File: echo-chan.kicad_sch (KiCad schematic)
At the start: 50 parts, among them J1 SJ1-3533NS, J2 USB_B, SW1 SW_Push, T1 Transformer_1P_1S, U1 JAMMA, U2 JAMMA, U3 AT90USB1286, U4 HD15, U6 THS7374, Y1 16MHz

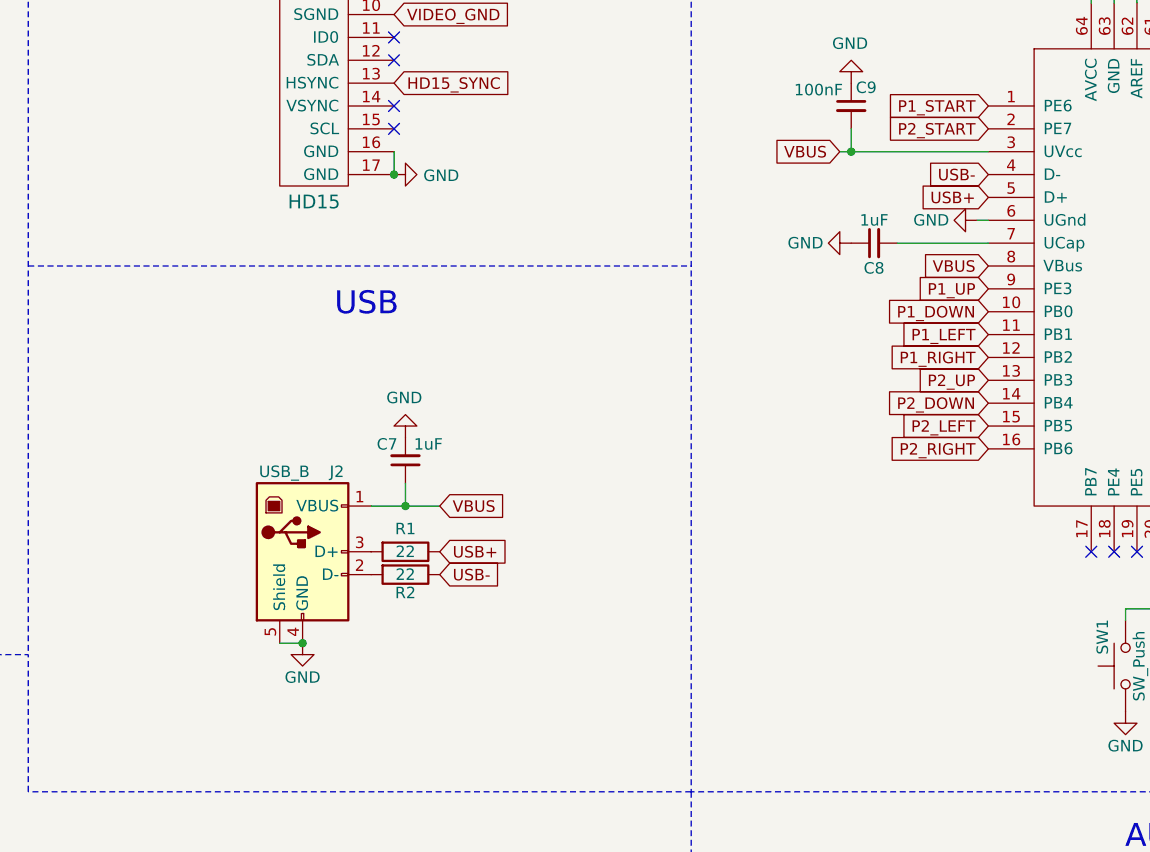
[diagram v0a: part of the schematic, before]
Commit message: [PCB] Routing done
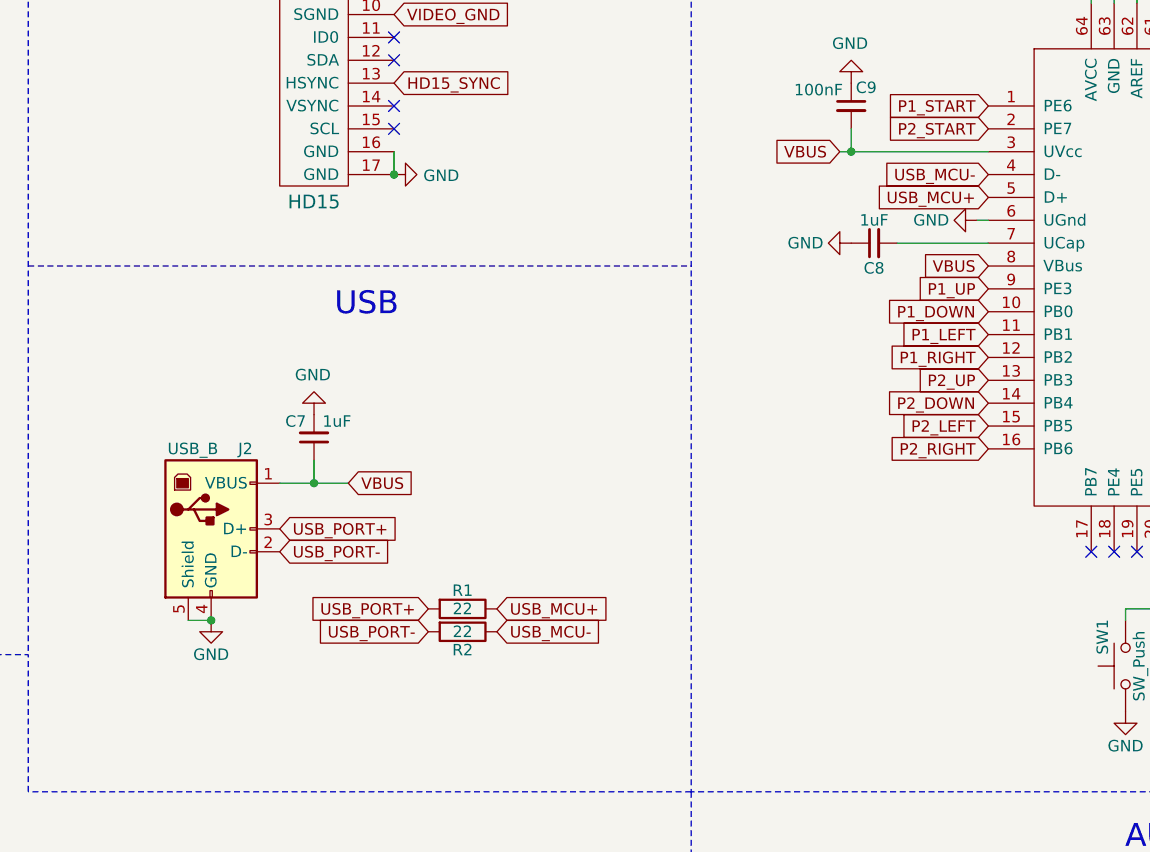
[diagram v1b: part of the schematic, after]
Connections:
- net USB_PORT+: now reaches J2.3 (D+), R1.2
- net USB_PORT-: now reaches J2.2 (D-), R2.2
- net USB+ renamed USB_MCU+
- net USB- renamed USB_MCU-
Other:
- moved on the sheet: C7, J2, R1, R2
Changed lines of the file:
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@@
 	)
 	(junction
-		(at 125.73 118.11)
+		(at 115.57 115.57)
 		(diameter 0)
 		(color 0 0 0 0)
@@
 	)
 	(junction
-		(at 137.16 102.87)
+		(at 127 100.33)
 		(diameter 0)
 		(color 0 0 0 0)
@@
 	(wire
 		(pts
-			(xy 137.16 102.87) (xy 140.97 102.87)
+			(xy 127 100.33) (xy 130.81 100.33)
 		)
 		(stroke
@@
 	(wire
 		(pts
-			(xy 133.35 102.87) (xy 137.16 102.87)
+			(xy 123.19 100.33) (xy 127 100.33)
 		)
 		(stroke
@@
 	(wire
 		(pts
-			(xy 123.19 118.11) (xy 125.73 118.11)
+			(xy 113.03 115.57) (xy 115.57 115.57)
 		)
 		(stroke
@@
 	(wire
 		(pts
-			(xy 137.16 100.33) (xy 137.16 102.87)
+			(xy 127 97.79) (xy 127 100.33)
 		)
 		(stroke
@@
 		)
 	)
+	(global_label "USB_PORT+"
+		(shape input)
+		(at 123.19 105.41 0)
+		(fields_autoplaced yes)
+		(effects
+			(font
+				(size 1.27 1.27)
+			)
+			(justify left)
+		)
+		(property "Intersheetrefs" "${INTERSHEET_REFS}"
+			(at 136.7091 105.41 0)
+			(effects
+				(font
+					(size 1.27 1.27)
+				)
+				(justify left)
+				(hide yes)
+			)
+		)
+	)
 	(global_label "P1_B4"
 		(shape input)
@@
 		)
 	)
-	(global_label "USB-"
+	(global_label "USB_MCU-"
 		(shape input)
-		(at 140.97 110.49 0)
+		(at 147.32 116.84 0)
 		(fields_autoplaced yes)
 		(effects
@@
 		)
 		(property "Intersheetrefs" "${INTERSHEET_REFS}"
-			(at 148.6834 110.49 0)
+			(at 160.0529 116.84 0)
 			(effects
 				(font
@@
 		)
 	)
-	(global_label "USB-"
+	(global_label "USB_MCU-"
 		(shape input)
 		(at 201.93 66.04 180)
@@
 		)
 		(property "Intersheetrefs" "${INTERSHEET_REFS}"
-			(at 194.2166 66.04 0)
+			(at 189.1971 66.04 0)
 			(effects
 				(font
@@
 		)
 	)
-	(global_label "USB+"
+	(global_label "USB_MCU+"
 		(shape input)
 		(at 201.93 68.58 180)
@@
 		)
 		(property "Intersheetrefs" "${INTERSHEET_REFS}"
-			(at 194.2166 68.58 0)
+			(at 189.1971 68.58 0)
 			(effects
 				(font
@@
 		)
 	)
+	(global_label "USB_PORT-"
+		(shape input)
+		(at 123.19 107.95 0)
+		(fields_autoplaced yes)
+		(effects
+			(font
+				(size 1.27 1.27)
+			)
+			(justify left)
+		)
+		(property "Intersheetrefs" "${INTERSHEET_REFS}"
+			(at 136.7091 107.95 0)
+			(effects
+				(font
+					(size 1.27 1.27)
+				)
+				(justify left)
+				(hide yes)
+			)
+		)
+	)
 	(global_label "COIN_LOCK_2"
 		(shape input)
@@
 	(global_label "VBUS"
 		(shape input)
-		(at 140.97 102.87 0)
+		(at 130.81 100.33 0)
 		(fields_autoplaced yes)
 		(effects
@@
 		)
 		(property "Intersheetrefs" "${INTERSHEET_REFS}"
-			(at 148.1996 102.87 0)
+			(at 138.0396 100.33 0)
 			(effects
 				(font
@@
 		)
 	)
+	(global_label "USB_PORT+"
+		(shape input)
+		(at 139.7 114.3 180)
+		(fields_autoplaced yes)
+		(effects
+			(font
+				(size 1.27 1.27)
+			)
+			(justify right)
+		)
+		(property "Intersheetrefs" "${INTERSHEET_REFS}"
+			(at 126.1809 114.3 0)
+			(effects
+				(font
+					(size 1.27 1.27)
+				)
+				(justify right)
+				(hide yes)
+			)
+		)
+	)
 	(global_label "P2_RIGHT"
 		(shape input)
@@
 		)
 	)
-	(global_label "USB+"
+	(global_label "USB_MCU+"
 		(shape input)
-		(at 140.97 107.95 0)
+		(at 147.32 114.3 0)
 		(fields_autoplaced yes)
 		(effects
@@
 		)
 		(property "Intersheetrefs" "${INTERSHEET_REFS}"
-			(at 148.6834 107.95 0)
+			(at 160.0529 114.3 0)
 			(effects
 				(font
@@
 		)
 	)
+	(global_label "USB_PORT-"
+		(shape input)
+		(at 139.7 116.84 180)
+		(fields_autoplaced yes)
+		(effects
+			(font
+				(size 1.27 1.27)
+			)
+			(justify right)
+		)
+		(property "Intersheetrefs" "${INTERSHEET_REFS}"
+			(at 126.1809 116.84 0)
+			(effects
+				(font
+					(size 1.27 1.27)
+				)
+				(justify right)
+				(hide yes)
+			)
+		)
+	)
 	(global_label "COIN_LOCK_2"
 		(shape input)
@@
 	(symbol
 		(lib_id "jamma-streamer-rescue:R-jamma-streamer-rescue")
-		(at 137.16 107.95 270)
+		(at 143.51 114.3 270)
 		(unit 1)
 		(exclude_from_sim no)
@@
 		(dnp no)
 		(property "Reference" "R1"
-			(at 137.16 105.41 90)
+			(at 143.51 112.268 90)
 			(effects
 				(font
@@
 		)
 		(property "Value" "22"
-			(at 137.16 107.95 90)
+			(at 143.51 114.3 90)
 			(effects
 				(font
@@
 		)
 		(property "Footprint" "Resistor_SMD:R_0805_2012Metric"
-			(at 137.16 106.172 90)
+			(at 143.51 112.522 90)
 			(effects
 				(font
@@
 		)
 		(property "Datasheet" ""
-			(at 137.16 107.95 0)
+			(at 143.51 114.3 0)
 			(effects
 				(font
@@
 		)
 		(property "Description" ""
-			(at 137.16 107.95 0)
+			(at 143.51 114.3 0)
 			(effects
 				(font
@@
 	(symbol
 		(lib_id "jamma-streamer-rescue:R-jamma-streamer-rescue")
-		(at 137.16 110.49 270)
+		(at 143.51 116.84 270)
 		(unit 1)
 		(exclude_from_sim no)
@@
 		(dnp no)
 		(property "Reference" "R2"
-			(at 137.16 112.522 90)
+			(at 143.51 118.872 90)
 			(effects
 				(font
@@
 		)
 		(property "Value" "22"
-			(at 137.16 110.49 90)
+			(at 143.51 116.84 90)
 			(effects
 				(font
@@
 		)
 		(property "Footprint" "Resistor_SMD:R_0805_2012Metric"
-			(at 137.16 108.712 90)
+			(at 143.51 115.062 90)
 			(effects
 				(font
@@
 		)
 		(property "Datasheet" ""
-			(at 137.16 110.49 0)
+			(at 143.51 116.84 0)
 			(effects
 				(font
@@
 		)
 		(property "Description" ""
-			(at 137.16 110.49 0)
+			(at 143.51 116.84 0)
 			(effects
 				(font
@@
 	(symbol
 		(lib_id "jamma-streamer-rescue:USB_B-Connector")
-		(at 125.73 107.95 0)
+		(at 115.57 105.41 0)
 		(unit 1)
 		(exclude_from_sim no)
@@
 		(dnp no)
 		(property "Reference" "J2"
-			(at 129.54 99.06 0)
+			(at 119.38 96.52 0)
 			(effects
 				(font
@@
 		)
 		(property "Value" "USB_B"
-			(at 123.698 99.06 0)
+			(at 113.538 96.52 0)
 			(effects
 				(font
@@
 		)
 		(property "Footprint" "Connector_USB:USB_B_OST_USB-B1HSxx_Horizontal"
-			(at 129.54 109.22 0)
+			(at 119.38 106.68 0)
 			(effects
 				(font
@@
 		)
 		(property "Datasheet" " ~"
-			(at 129.54 109.22 0)
+			(at 119.38 106.68 0)
 			(effects
 				(font
@@
 		)
 		(property "Description" ""
-			(at 125.73 107.95 0)
+			(at 115.57 105.41 0)
 			(effects
 				(font
@@
 	(symbol
 		(lib_id "jamma-streamer-rescue:GND-jamma-streamer-rescue")
-		(at 125.73 118.11 0)
+		(at 115.57 115.57 0)
 		(unit 1)
 		(exclude_from_sim no)
@@
 		(dnp no)
 		(property "Reference" "#PWR0110"
-			(at 125.73 124.46 0)
+			(at 115.57 121.92 0)
 			(effects
 				(font
@@
 		)
 		(property "Value" "GND"
-			(at 125.73 121.92 0)
+			(at 115.57 119.38 0)
 			(effects
 				(font
@@
 		)
 		(property "Footprint" ""
-			(at 125.73 118.11 0)
+			(at 115.57 115.57 0)
 			(effects
 				(font
@@
 		)
 		(property "Datasheet" ""
-			(at 125.73 118.11 0)
+			(at 115.57 115.57 0)
 			(effects
 				(font
@@
 		)
 		(property "Description" ""
-			(at 125.73 118.11 0)
+			(at 115.57 115.57 0)
 			(effects
 				(font
@@
 	(symbol
 		(lib_id "jamma-streamer-rescue:GND-jamma-streamer-rescue")
-		(at 137.16 95.25 180)
+		(at 127 92.71 180)
 		(unit 1)
 		(exclude_from_sim no)
@@
 		(dnp no)
 		(property "Reference" "#PWR01"
-			(at 137.16 88.9 0)
+			(at 127 86.36 0)
 			(effects
 				(font
@@
 		)
 		(property "Value" "GND"
-			(at 137.033 90.8558 0)
+			(at 126.873 88.3158 0)
 			(effects
 				(font
@@
 		)
 		(property "Footprint" ""
-			(at 137.16 95.25 0)
+			(at 127 92.71 0)
 			(effects
 				(font
@@
 		)
 		(property "Datasheet" ""
-			(at 137.16 95.25 0)
+			(at 127 92.71 0)
 			(effects
 				(font
@@
 		)
 		(property "Description" ""
-			(at 137.16 95.25 0)
+			(at 127 92.71 0)
 			(effects
 				(font
@@
 	(symbol
 		(lib_id "Device:C_Small")
-		(at 137.16 97.79 180)
+		(at 127 95.25 180)
 		(unit 1)
 		(exclude_from_sim no)
@@
 		(dnp no)
 		(property "Reference" "C7"
-			(at 135.128 96.012 0)
+			(at 124.968 93.472 0)
 			(effects
 				(font
@@
 		)
 		(property "Value" "1uF"
-			(at 139.7 96.012 0)
+			(at 129.54 93.472 0)
 			(effects
 				(font
@@
 		)
 		(property "Footprint" "Capacitor_SMD:C_0805_2012Metric"
-			(at 137.16 97.79 0)
+			(at 127 95.25 0)
 			(effects
 				(font
@@
 		)
 		(property "Datasheet" "~"
-			(at 137.16 97.79 0)
+			(at 127 95.25 0)
 			(effects
 				(font
@@
 		)
 		(property "Description" ""
-			(at 137.16 97.79 0)
+			(at 127 95.25 0)
 			(effects
 				(font
